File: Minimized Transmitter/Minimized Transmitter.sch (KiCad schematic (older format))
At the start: 10 parts, among them J2 Conn_01x02_Male, J4 Conn_01x05_Male, SW1 SW_Push, U1 LPC824M201JHI33, U2 RFM69HCW

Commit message: Done except for deciding on a power switch
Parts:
- added J1: Conn_01x03_Male, my_foot_prints:SlideSwitch_SMD_PN#COM-10860, symbol Connector:Conn_01x03_Male
- J2: footprint Connector_PinHeader_2.54mm:PinHeader_1x02_P2.54mm_Vertical -> my_foot_prints:2_pad_sufacemount
- U2: symbol Minimized-Transmitter-rescue:RFM69HCW-Transmitter~board-rescue -> Minimized-Transmitter-rescue:RFM69HCW-Transmitter_board-rescue
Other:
- moved on the sheet: BT1
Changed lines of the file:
@@
 L Device:Battery_Cell BT1
 U 1 1 5BDB3AA6
-P 6500 1800
-F 0 "BT1" V 6700 1850 50  0000 L CNN
-F 1 "Battery_Cell" V 6618 1805 50  0000 L CNN
-F 2 "my_foot_prints:PRT-11892" V 6500 1860 50  0001 C CNN
-F 3 "~" V 6500 1860 50  0001 C CNN
-	1    6500 1800
+P 5250 3400
+F 0 "BT1" V 5450 3450 50  0000 L CNN
+F 1 "Battery_Cell" V 5368 3405 50  0000 L CNN
+F 2 "my_foot_prints:PRT-11892" V 5250 3460 50  0001 C CNN
+F 3 "~" V 5250 3460 50  0001 C CNN
+	1    5250 3400
 	0    -1   -1   0
 $EndComp
@@
 L power:GND #PWR0105
 U 1 1 5BDB3BBB
-P 6600 1800
-F 0 "#PWR0105" H 6600 1550 50  0001 C CNN
-F 1 "GND" H 6605 1627 50  0000 C CNN
-F 2 "" H 6600 1800 50  0001 C CNN
-F 3 "" H 6600 1800 50  0001 C CNN
-	1    6600 1800
-	0    -1   -1   0
+P 5350 3400
+F 0 "#PWR0105" H 5350 3150 50  0001 C CNN
+F 1 "GND" H 5355 3227 50  0000 C CNN
+F 2 "" H 5350 3400 50  0001 C CNN
+F 3 "" H 5350 3400 50  0001 C CNN
+	1    5350 3400
+	1    0    0    -1
 $EndComp
 Text GLabel 3700 4500 2    50   Input ~ 0
@@
 	1    0    0    -1
 $EndComp
-Text GLabel 3200 1700 2    50   Input ~ 0
+Text GLabel 1800 1700 0    50   Input ~ 0
 LED
 Text GLabel 1800 1800 0    50   Input ~ 0
@@
 F 0 "J2" H 5073 2430 50  0000 R CNN
 F 1 "Conn_01x02_Male" H 5073 2521 50  0000 R CNN
-F 2 "Connector_PinHeader_2.54mm:PinHeader_1x02_P2.54mm_Vertical" H 5100 2550 50  0001 C CNN
+F 2 "my_foot_prints:2_pad_sufacemount" H 5100 2550 50  0001 C CNN
 F 3 "~" H 5100 2550 50  0001 C CNN
 	1    5100 2550
@@
 $EndComp
 $Comp
-L Minimized-Transmitter-rescue:RFM69HCW-Transmitter~board-rescue U2
+L Minimized-Transmitter-rescue:RFM69HCW-Transmitter_board-rescue U2
 U 1 1 5C15B19A
 P 6900 4500
@@
 L power:+3V3 #PWR0106
 U 1 1 5BDB3C26
-P 6200 1800
-F 0 "#PWR0106" H 6200 1650 50  0001 C CNN
-F 1 "+3V3" V 6215 1928 50  0000 L CNN
-F 2 "" H 6200 1800 50  0001 C CNN
-F 3 "" H 6200 1800 50  0001 C CNN
-	1    6200 1800
-	-1   0    0    1
-$EndComp
-Wire Wire Line
-	6200 1800 6300 1800
+P 4700 3500
+F 0 "#PWR0106" H 4700 3350 50  0001 C CNN
+F 1 "+3V3" V 4715 3628 50  0000 L CNN
+F 2 "" H 4700 3500 50  0001 C CNN
+F 3 "" H 4700 3500 50  0001 C CNN
+	1    4700 3500
+	0    1    1    0
+$EndComp
 $Comp
 L Switch:SW_Push SW1
@@
 Text Notes 4950 1300 0    50   ~ 0
 LED
-Text Notes 6250 1550 0    50   ~ 0
+Text Notes 5000 3150 0    50   ~ 0
 Battery
 Text Notes 6800 3850 0    50   ~ 0
@@
 Text Notes 7550 2900 0    50   ~ 0
 Programable Button\n
+$Comp
+L Connector:Conn_01x03_Male J1
+U 1 1 5C2FB3B8
+P 4500 3500
+F 0 "J1" H 4606 3778 50  0000 C CNN
+F 1 "Conn_01x03_Male" H 4606 3687 50  0000 C CNN
+F 2 "my_foot_prints:SlideSwitch_SMD_PN#COM-10860" H 4500 3500 50  0001 C CNN
+F 3 "~" H 4500 3500 50  0001 C CNN
+	1    4500 3500
+	1    0    0    -1
+$EndComp
+Wire Wire Line
+	5050 3400 4700 3400
+$Comp
+L power:GND #PWR0114
+U 1 1 5C2FB7A8
+P 4700 3600
+F 0 "#PWR0114" H 4700 3350 50  0001 C CNN
+F 1 "GND" H 4705 3427 50  0000 C CNN
+F 2 "" H 4700 3600 50  0001 C CNN
+F 3 "" H 4700 3600 50  0001 C CNN
+	1    4700 3600
+	1    0    0    -1
+$EndComp
 $EndSCHEMATC

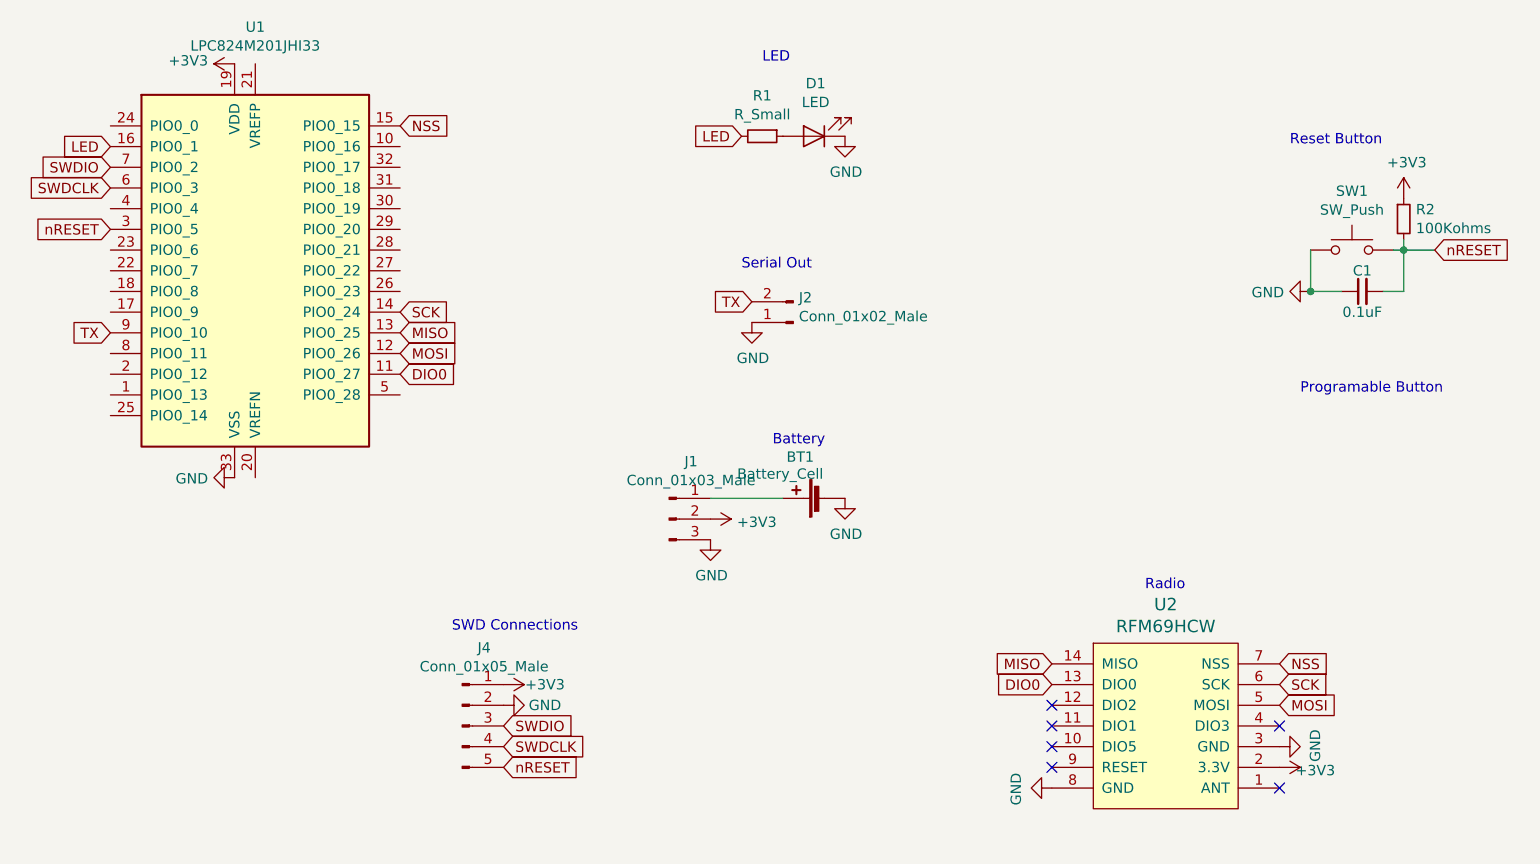
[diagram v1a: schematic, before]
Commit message: unsaved files
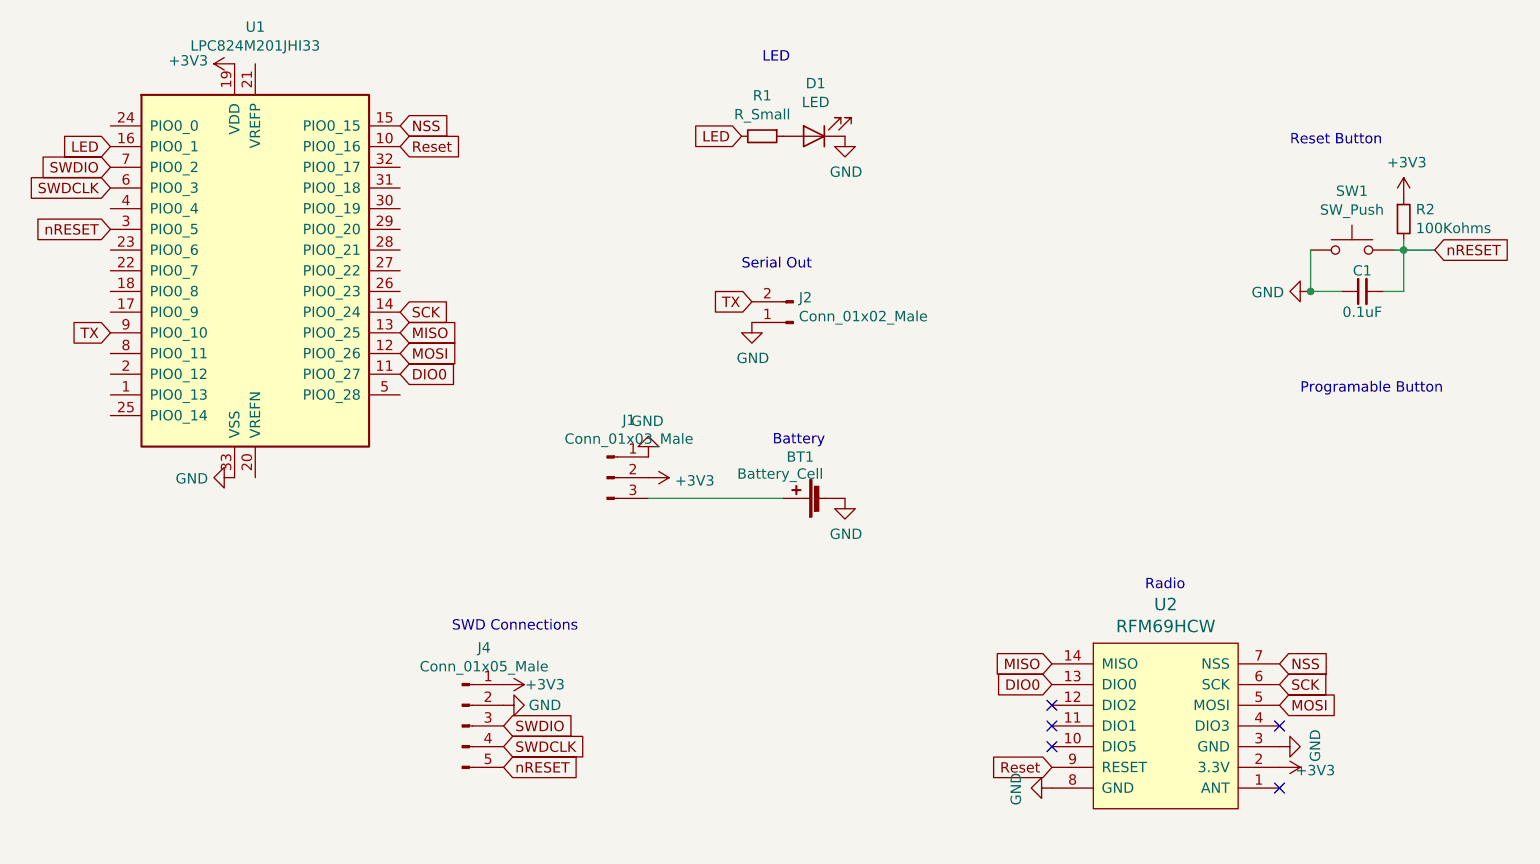
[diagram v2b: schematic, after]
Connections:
- net GND: now also J1.1 (Pin_1); no longer J1.3 (Pin_3)
- net Reset: now reaches U1.10 (PIO0_16)
- net Reset: now also U2.9 (RESET)
- net at BT1.1 (+): now also J1.3 (Pin_3); no longer J1.1 (Pin_1)
- no-connect marks 6 -> 5
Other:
- moved on the sheet: J1
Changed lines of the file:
@@
 LED
 NoConn ~ 7450 4500
-NoConn ~ 6350 4700
 NoConn ~ 6350 4600
 NoConn ~ 6350 4500
@@
 L power:+3V3 #PWR0106
 U 1 1 5BDB3C26
-P 4700 3500
-F 0 "#PWR0106" H 4700 3350 50  0001 C CNN
-F 1 "+3V3" V 4715 3628 50  0000 L CNN
-F 2 "" H 4700 3500 50  0001 C CNN
-F 3 "" H 4700 3500 50  0001 C CNN
-	1    4700 3500
+P 4400 3300
+F 0 "#PWR0106" H 4400 3150 50  0001 C CNN
+F 1 "+3V3" V 4415 3428 50  0000 L CNN
+F 2 "" H 4400 3300 50  0001 C CNN
+F 3 "" H 4400 3300 50  0001 C CNN
+	1    4400 3300
 	0    1    1    0
 $EndComp
@@
 L Connector:Conn_01x03_Male J1
 U 1 1 5C2FB3B8
-P 4500 3500
-F 0 "J1" H 4606 3778 50  0000 C CNN
-F 1 "Conn_01x03_Male" H 4606 3687 50  0000 C CNN
-F 2 "my_foot_prints:SlideSwitch_SMD_PN#COM-10860" H 4500 3500 50  0001 C CNN
-F 3 "~" H 4500 3500 50  0001 C CNN
-	1    4500 3500
+P 4200 3300
+F 0 "J1" H 4306 3578 50  0000 C CNN
+F 1 "Conn_01x03_Male" H 4306 3487 50  0000 C CNN
+F 2 "my_foot_prints:SlideSwitch_SMD_PN#COM-10860" H 4200 3300 50  0001 C CNN
+F 3 "~" H 4200 3300 50  0001 C CNN
+	1    4200 3300
 	1    0    0    -1
 $EndComp
-Wire Wire Line
-	5050 3400 4700 3400
 $Comp
 L power:GND #PWR0114
 U 1 1 5C2FB7A8
-P 4700 3600
-F 0 "#PWR0114" H 4700 3350 50  0001 C CNN
-F 1 "GND" H 4705 3427 50  0000 C CNN
-F 2 "" H 4700 3600 50  0001 C CNN
-F 3 "" H 4700 3600 50  0001 C CNN
-	1    4700 3600
-	1    0    0    -1
+P 4400 3200
+F 0 "#PWR0114" H 4400 2950 50  0001 C CNN
+F 1 "GND" H 4405 3027 50  0000 C CNN
+F 2 "" H 4400 3200 50  0001 C CNN
+F 3 "" H 4400 3200 50  0001 C CNN
+	1    4400 3200
+	-1   0    0    1
 $EndComp
+Text GLabel 6350 4700 0    50   Input ~ 0
+Reset
+Text GLabel 3200 1700 2    50   Input ~ 0
+Reset
+Wire Wire Line
+	4400 3400 5050 3400
 $EndSCHEMATC
